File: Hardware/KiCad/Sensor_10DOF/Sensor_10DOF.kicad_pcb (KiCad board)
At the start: 2 copper layers, 38.5 x 30.1 mm, 24 parts, among them J1 Conn_01x04, U1 BMI160, U2 BME280, U3 LSM303AGR, U4 WeMos_D1_mini, U6 LP2985-3.3

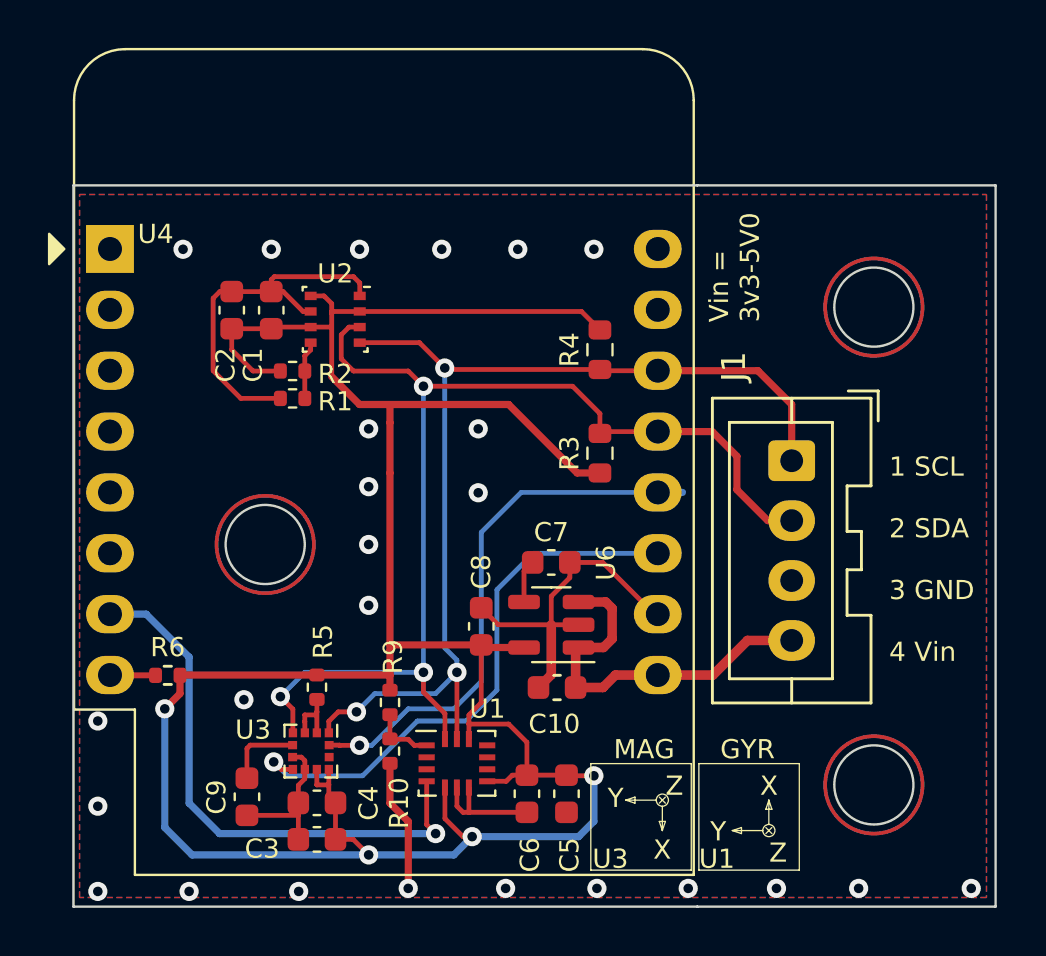
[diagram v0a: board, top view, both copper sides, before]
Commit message: fix gerber
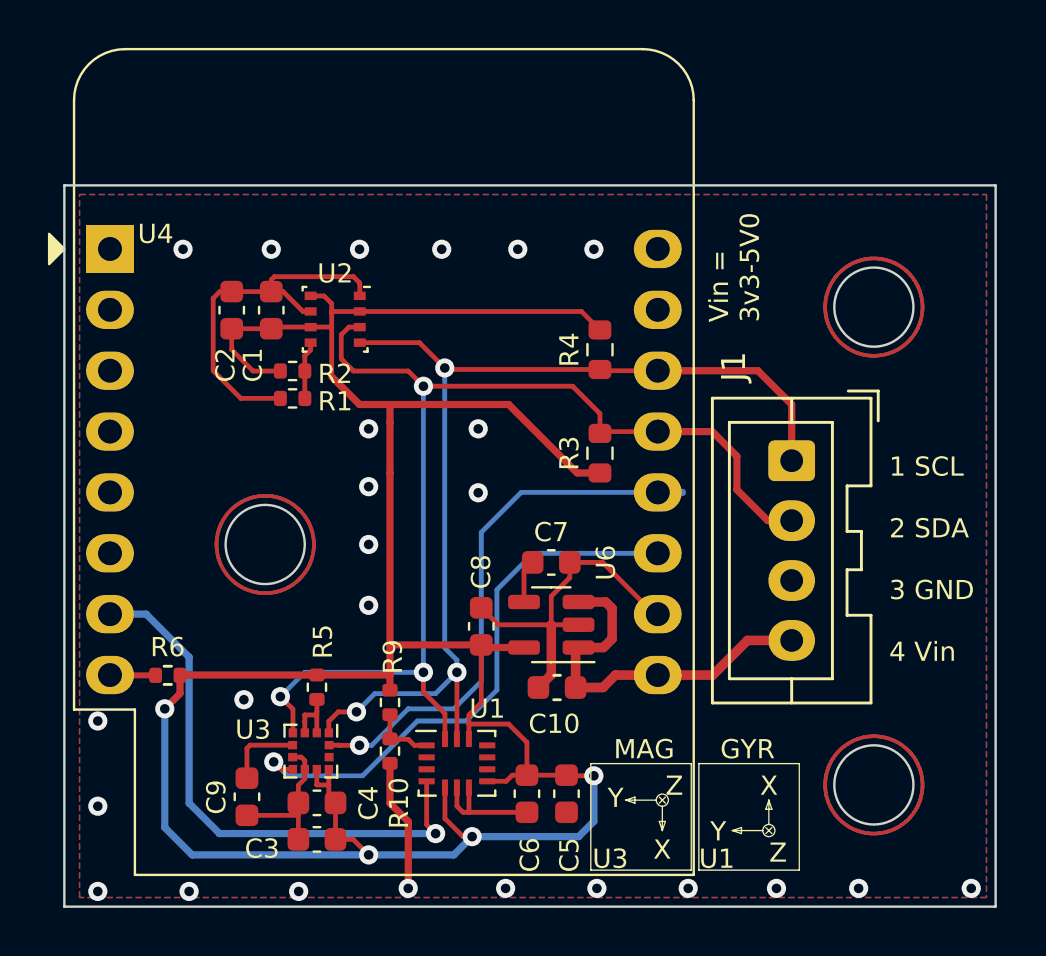
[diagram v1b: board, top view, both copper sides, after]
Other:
- board size 38.5 x 30.1 mm -> 38.9 x 30.1 mm
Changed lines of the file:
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@@
     (pad_to_mask_clearance 0)
     (pcbplotparams
-      (layerselection 0x00010fc_ffffffff)
+      (layerselection 0x0000000_7fffffff)
       (plot_on_all_layers_selection 0x0001120_00000001)
       (disableapertmacros false)
@@
       (sketchpadsonfab false)
       (subtractmaskfromsilk true)
-      (outputformat 1)
+      (outputformat 4)
       (mirror false)
       (drillshape 0)
       (scaleselection 1)
-      (outputdirectory "gerber/")
+      (outputdirectory "./")
     )
   )
@@
     (property "ki_description" "Resistor")
     (property "ki_keywords" "R res resistor")
-    (attr smd)
+    (attr smd exclude_from_pos_files exclude_from_bom allow_missing_courtyard)
     (fp_text reference "R2" (at 1.778 0.127) (layer "F.SilkS")
         (effects (font (size 0.8 0.8) (thickness 0.15)))
@@
     (property "ki_description" "32-bit microcontroller module with WiFi")
     (property "ki_keywords" "ESP8266 WiFi microcontroller ESP8266EX")
-    (attr through_hole)
+    (attr through_hole exclude_from_pos_files exclude_from_bom allow_missing_courtyard)
     (fp_text reference "U4" (at 1.905 -0.622) (layer "F.SilkS")
         (effects (font (size 0.8 0.8) (thickness 0.15)))
@@
     (property "ki_description" "Resistor")
     (property "ki_keywords" "R res resistor")
-    (attr smd)
+    (attr smd exclude_from_pos_files exclude_from_bom allow_missing_courtyard)
     (fp_text reference "R9" (at -1.905 -0.127 90) (layer "F.SilkS")
         (effects (font (size 0.8 0.8) (thickness 0.15)))
@@
     (property "ki_description" "Resistor")
     (property "ki_keywords" "R res resistor")
-    (attr smd)
+    (attr smd exclude_from_pos_files exclude_from_bom allow_missing_courtyard)
     (fp_text reference "R6" (at 0 -1.17) (layer "F.SilkS")
         (effects (font (size 0.8 0.8) (thickness 0.15)))
@@
     (property "ki_description" "Generic connector, single row, 01x04, script generated (kicad-library-utils/schlib/autogen/connector/)")
     (property "ki_keywords" "connector")
-    (attr through_hole)
+    (attr through_hole exclude_from_pos_files exclude_from_bom allow_missing_courtyard)
     (fp_text reference "J1" (at -3.93 2.413 90) (layer "F.SilkS")
         (effects (font (size 1 1) (thickness 0.15)))
@@
   (gr_circle (center 109.982 96.774) (end 109.982 95.123)
     (stroke (width 0.1) (type default)) (fill none) (layer "Edge.Cuts"))
-  (gr_line (start 128.016 111.887) (end 101.981 111.887)
+  (gr_line (start 140.462 111.887) (end 101.6 111.887)
     (stroke (width 0.1) (type default)) (layer "Edge.Cuts"))
-  (gr_line (start 101.981 81.788) (end 128.016 81.788)
-    (stroke (width 0.1) (type default)) (layer "Edge.Cuts"))
-  (gr_line (start 128.016 111.887) (end 140.462 111.887)
+  (gr_line (start 101.6 81.788) (end 140.462 81.788)
     (stroke (width 0.1) (type default)) (layer "Edge.Cuts"))
   (gr_circle (center 135.382 106.807) (end 137.033 106.807)
@@
   (gr_line (start 140.462 81.788) (end 140.462 111.887)
     (stroke (width 0.1) (type default)) (layer "Edge.Cuts"))
-  (gr_line (start 101.981 111.887) (end 101.981 81.788)
-    (stroke (width 0.1) (type default)) (layer "Edge.Cuts"))
-  (gr_line (start 128.016 81.788) (end 140.462 81.788)
+  (gr_line (start 101.6 111.887) (end 101.6 81.788)
     (stroke (width 0.1) (type default)) (layer "Edge.Cuts"))
   (gr_text "VBUS\n\nGND\n\nINT_M\n\nINT_XL\n\nSDA\n\nSCL\n\nRXD\n\nTXD\n" (at 121.412 83.693 180) (layer "B.SilkS")
@@
   )
   (dimension (type aligned) (layer "Dwgs.User")
-    (pts (xy 109.982 96.774) (xy 109.982 81.788))
-    (height -11.684)
-    (gr_text "14.99 mm" (at 97.148 89.281 90) (layer "Dwgs.User")
+    (pts (xy 140.462 81.788) (xy 140.462 111.887))
+    (height -7.493)
+    (gr_text "30.10 mm" (at 146.805 96.8375 90) (layer "Dwgs.User")
       (effects (font (size 1 1) (thickness 0.15)))
     )
@@
   )
   (dimension (type aligned) (layer "Dwgs.User")
-    (pts (xy 109.982 96.774) (xy 101.981 96.774))
-    (height 26.67)
-    (gr_text "8.00 mm" (at 105.9815 68.954) (layer "Dwgs.User")
+    (pts (xy 109.982 96.774) (xy 109.982 81.788))
+    (height -11.049)
+    (gr_text "14.99 mm" (at 97.783 89.281 90) (layer "Dwgs.User")
       (effects (font (size 1 1) (thickness 0.15)))
     )
@@
   )
   (dimension (type aligned) (layer "Dwgs.User")
-    (pts (xy 101.981 81.788) (xy 140.462 81.788))
-    (height -8.001)
-    (gr_text "38.4810 mm" (at 121.2215 71.987) (layer "Dwgs.User")
-      (effects (font (size 1.5 1.5) (thickness 0.3)))
-    )
-    (format (prefix "") (suffix "") (units 3) (units_format 1) (precision 4))
-    (style (thickness 0.2) (arrow_length 1.27) (text_position_mode 0) (extension_height 0.58642) (extension_offset 0.5) keep_text_aligned)
+    (pts (xy 135.382 86.868) (xy 140.462 86.868))
+    (height -7.874)
+    (gr_text "5.08 mm" (at 139.954 77.724) (layer "Dwgs.User")
+      (effects (font (size 1 1) (thickness 0.15)))
+    )
+    (format (prefix "") (suffix "") (units 3) (units_format 1) (precision 2))
+    (style (thickness 0.15) (arrow_length 1.27) (text_position_mode 2) (extension_height 0.58642) (extension_offset 0.5) keep_text_aligned)
+  )
+  (dimension (type aligned) (layer "Dwgs.User")
+    (pts (xy 101.6 81.788) (xy 140.462 81.788))
+    (height -10.033)
+    (gr_text "38.86 mm" (at 121.031 70.605) (layer "Dwgs.User")
+      (effects (font (size 1 1) (thickness 0.15)))
+    )
+    (format (prefix "") (suffix "") (units 3) (units_format 1) (precision 2))
+    (style (thickness 0.15) (arrow_length 1.27) (text_position_mode 0) (extension_height 0.58642) (extension_offset 0.5) keep_text_aligned)
+  )
+  (dimension (type aligned) (layer "Dwgs.User")
+    (pts (xy 109.982 96.774) (xy 101.6 96.774))
+    (height 21.971)
+    (gr_text "8.38 mm" (at 105.791 73.653) (layer "Dwgs.User")
+      (effects (font (size 1 1) (thickness 0.15)))
+    )
+    (format (prefix "") (suffix "") (units 3) (units_format 1) (precision 2))
+    (style (thickness 0.15) (arrow_length 1.27) (text_position_mode 0) (extension_height 0.58642) (extension_offset 0.5) keep_text_aligned)
   )
   (dimension (type aligned) (layer "Dwgs.User")
     (pts (xy 135.382 86.868) (xy 135.382 81.788))
     (height 8.636)
-    (gr_text "5.08 mm" (at 143.891 77.978 90) (layer "Dwgs.User")
+    (gr_text "5.08 mm" (at 142.621 82.296 90) (layer "Dwgs.User")
       (effects (font (size 1 1) (thickness 0.15)))
     )
-    (format (prefix "") (suffix "") (units 3) (units_format 1) (precision 2))
-    (style (thickness 0.15) (arrow_length 1.27) (text_position_mode 2) (extension_height 0.58642) (extension_offset 0.5) keep_text_aligned)
-  )
-  (dimension (type aligned) (layer "Dwgs.User")
-    (pts (xy 135.382 86.868) (xy 140.462 86.868))
-    (height -8.89)
-    (gr_text "5.08 mm" (at 138.43 76.581) (layer "Dwgs.User")
-      (effects (font (size 1 1) (thickness 0.15)))
-    )
-    (format (prefix "") (suffix "") (units 3) (units_format 1) (precision 2))
-    (style (thickness 0.15) (arrow_length 1.27) (text_position_mode 2) (extension_height 0.58642) (extension_offset 0.5) keep_text_aligned)
-  )
-  (dimension (type aligned) (layer "Dwgs.User")
-    (pts (xy 135.382 106.807) (xy 140.462 106.807))
-    (height 9.525)
-    (gr_text "5.08 mm" (at 138.049 118.364) (layer "Dwgs.User")
-      (effects (font (size 1 1) (thickness 0.15)))
-    )
-    (format (prefix "") (suffix "") (units 3) (units_format 1) (precision 2))
-    (style (thickness 0.15) (arrow_length 1.27) (text_position_mode 2) (extension_height 0.58642) (extension_offset 0.5) keep_text_aligned)
-  )
-  (dimension (type aligned) (layer "Dwgs.User")
-    (pts (xy 140.462 111.887) (xy 140.462 81.788))
-    (height 6.858)
-    (gr_text "30.0990 mm" (at 146.17 96.8375 90) (layer "Dwgs.User")
-      (effects (font (size 1 1) (thickness 0.15)))
-    )
-    (format (prefix "") (suffix "") (units 3) (units_format 1) (precision 4))
-    (style (thickness 0.15) (arrow_length 1.27) (text_position_mode 0) (extension_height 0.58642) (extension_offset 0.5) keep_text_aligned)
-  )
-  (dimension (type aligned) (layer "Dwgs.User")
-    (pts (xy 135.382 106.807) (xy 135.382 111.887))
-    (height -8.509)
-    (gr_text "5.08 mm" (at 145.542 108.331 90) (layer "Dwgs.User")
-      (effects (font (size 1 1) (thickness 0.15)))
-    )

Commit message: bestückungsplan erstellt
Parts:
- R2, R6, R9: value N.P. -> DNP
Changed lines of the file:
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@@
     (pad_to_mask_clearance 0)
     (pcbplotparams
-      (layerselection 0x0000000_7fffffff)
-      (plot_on_all_layers_selection 0x0001120_00000001)
+      (layerselection 0x0000020_7ffffffe)
+      (plot_on_all_layers_selection 0x0001020_00000000)
       (disableapertmacros false)
       (usegerberextensions true)
@@
         (effects (font (size 0.8 0.8) (thickness 0.15)))
     )
-    (fp_text value "10uF" (at 0 1.43) (layer "F.Fab")
+    (fp_text value "10uF" (at -3.048 -0.013) (layer "F.Fab")
         (effects (font (size 0.8 0.8) (thickness 0.15)))
     )
@@
         (effects (font (size 0.8 0.8) (thickness 0.15)))
     )
-    (fp_text value "0R0" (at 0 1.17) (layer "F.Fab")
+    (fp_text value "0R0" (at 2.159 1.016) (layer "F.Fab")
         (effects (font (size 0.8 0.8) (thickness 0.15)))
     )
@@
         (effects (font (size 0.8 0.8) (thickness 0.15)))
     )
-    (fp_text value "LP2985-3.3" (at 0 2.4) (layer "F.Fab")
+    (fp_text value "LP2985-3.3" (at 5.588 2.334) (layer "F.Fab")
         (effects (font (size 0.8 0.8) (thickness 0.15)))
     )
@@
         (effects (font (size 0.8 0.8) (thickness 0.15)))
     )
-    (fp_text value "10nF" (at 0 1.43) (layer "F.Fab")
+    (fp_text value "10nF" (at 0 -1.257) (layer "F.Fab")
         (effects (font (size 0.8 0.8) (thickness 0.15)))
     )
@@
     (property "ki_description" "Resistor")
     (property "ki_keywords" "R res resistor")
-    (attr smd exclude_from_pos_files exclude_from_bom allow_missing_courtyard)
+    (attr smd exclude_from_pos_files allow_missing_courtyard)
     (fp_text reference "R2" (at 1.778 0.127) (layer "F.SilkS")
         (effects (font (size 0.8 0.8) (thickness 0.15)))
     )
-    (fp_text value "N.P." (at 0 1.17) (layer "F.Fab")
+    (fp_text value "DNP" (at -2.159 1.27) (layer "F.Fab")
         (effects (font (size 0.8 0.8) (thickness 0.15)))
     )
@@
     (property "ki_description" "32-bit microcontroller module with WiFi")
     (property "ki_keywords" "ESP8266 WiFi microcontroller ESP8266EX")
-    (attr through_hole exclude_from_pos_files exclude_from_bom allow_missing_courtyard)
+    (attr through_hole exclude_from_pos_files allow_missing_courtyard)
     (fp_text reference "U4" (at 1.905 -0.622) (layer "F.SilkS")
         (effects (font (size 0.8 0.8) (thickness 0.15)))
     )
-    (fp_text value "WeMos_D1_mini" (at 11.7 0) (layer "F.Fab")
+    (fp_text value "WeMos_D1_mini" (at 8.128 -0.876) (layer "F.Fab")
         (effects (font (size 0.8 0.8) (thickness 0.15)))
     )
@@
         (effects (font (size 0.8 0.8) (thickness 0.15)))
     )
-    (fp_text user "${REFERENCE}" (at 11.43 10) (layer "F.Fab")
+    (fp_text user "${REFERENCE}" (at 1.905 -0.876) (layer "F.Fab")
         (effects (font (size 0.8 0.8) (thickness 0.15)))
     )
@@
         (effects (font (size 0.8 0.8) (thickness 0.15)))
     )
-    (fp_text value "1u" (at 0 1.43) (layer "F.Fab")
+    (fp_text value "1u" (at -2.426 -0.508) (layer "F.Fab")
         (effects (font (size 1 1) (thickness 0.15)))
     )
@@
         (effects (font (size 0.8 0.8) (thickness 0.15)))
     )
-    (fp_text value "0R0" (at 2.286 -0.127 90) (layer "F.Fab") hide
+    (fp_text value "0R0" (at 0.14 0.889 90) (layer "F.Fab")
         (effects (font (size 0.8 0.8) (thickness 0.15)))
     )
@@
         (effects (font (size 0.8 0.8) (thickness 0.15)))
     )
-    (fp_text value "100nF" (at 0 1.43 90) (layer "F.Fab")
+    (fp_text value "100nF" (at 0.127 -1.397 90) (layer "F.Fab")
         (effects (font (size 0.8 0.8) (thickness 0.15)))
     )
@@
     (property "ki_description" "Resistor")
     (property "ki_keywords" "R res resistor")
-    (attr smd exclude_from_pos_files exclude_from_bom allow_missing_courtyard)
+    (attr smd exclude_from_pos_files allow_missing_courtyard)
     (fp_text reference "R9" (at -1.905 -0.127 90) (layer "F.SilkS")
         (effects (font (size 0.8 0.8) (thickness 0.15)))
     )
-    (fp_text value "N.P." (at 0 1.17 90) (layer "F.Fab") hide
+    (fp_text value "DNP" (at -1.511 0.889 -90) (layer "F.Fab")
         (effects (font (size 0.8 0.8) (thickness 0.15)))
     )
@@
         (effects (font (size 0.8 0.8) (thickness 0.15)))
     )
-    (fp_text value "0R0" (at 0 1.17 90) (layer "F.Fab")
+    (fp_text value "0R0" (at -2.146 -0.127 90) (layer "F.Fab")
         (effects (font (size 0.8 0.8) (thickness 0.15)))
     )
@@
         (effects (font (size 0.8 0.8) (thickness 0.15)))
     )
-    (fp_text value "220nF" (at 0 1.43 90) (layer "F.Fab")
+    (fp_text value "220nF" (at 0 1.27 90) (layer "F.Fab")
         (effects (font (size 0.8 0.8) (thickness 0.15)))
     )
@@
         (effects (font (size 0.8 0.8) (thickness 0.15)))
     )
-    (fp_text value "100nF" (at 0 1.43 90) (layer "F.Fab")
+    (fp_text value "100nF" (at 2.299 0) (layer "F.Fab")
         (effects (font (size 0.8 0.8) (thickness 0.15)))
     )
@@
     (property "ki_description" "Resistor")
     (property "ki_keywords" "R res resistor")
-    (attr smd exclude_from_pos_files exclude_from_bom allow_missing_courtyard)
+    (attr smd exclude_from_pos_files allow_missing_courtyard)
     (fp_text reference "R6" (at 0 -1.17) (layer "F.SilkS")
         (effects (font (size 0.8 0.8) (thickness 0.15)))
     )
-    (fp_text value "N.P." (at 0 1.17) (layer "F.Fab")
-        (effects (font (size 1 1) (thickness 0.15)))
+    (fp_text value "DNP" (at 2.415 -0.381) (layer "F.Fab")
+        (effects (font (size 0.8 0.8) (thickness 0.15)))
     )
     (fp_text user "${REFERENCE}" (at 0 0) (layer "F.Fab")
@@
         (effects (font (size 0.8 0.8) (thickness 0.15)))
     )
-    (fp_text value "BMI160" (at 0 2.5) (layer "F.Fab")
+    (fp_text value "BMI160" (at 0.381 -2.019) (layer "F.Fab")
         (effects (font (size 0.8 0.8) (thickness 0.15)))
     )
@@
         (effects (font (size 0.8 0.8) (thickness 0.15)))
     )
-    (fp_text value "4K7" (at 0 1.43 90) (layer "F.Fab")
+    (fp_text value "4K7" (at 0 -1.27 90) (layer "F.Fab")
         (effects (font (size 0.8 0.8) (thickness 0.15)))
     )
@@
     (property "ki_description" "Generic connector, single row, 01x04, script generated (kicad-library-utils/schlib/autogen/connector/)")
     (property "ki_keywords" "connector")
-    (attr through_hole exclude_from_pos_files exclude_from_bom allow_missing_courtyard)
+    (attr through_hole exclude_from_pos_files allow_missing_courtyard)
     (fp_text reference "J1" (at -3.93 2.413 90) (layer "F.SilkS")
         (effects (font (size 1 1) (thickness 0.15)))
     )
-    (fp_text value "Conn_01x04" (at 3.75 4.4 90) (layer "F.Fab")
+    (fp_text value "Conn_01x04" (at 3.877 -4.572 90) (layer "F.Fab")
         (effects (font (size 1 1) (thickness 0.15)))
     )
@@
         (effects (font (size 0.8 0.8) (thickness 0.15)))
     )
-    (fp_text value "100nF" (at 0 1.43 90) (layer "F.Fab")
+    (fp_text value "100nF" (at -2.019 -0.381 -180) (layer "F.Fab")
         (effects (font (size 0.8 0.8) (thickness 0.15)))
     )
@@
         (effects (font (size 0.8 0.8) (thickness 0.15)))
     )
-    (fp_text value "BME280" (at 0.015 2.535 90) (layer "F.Fab")
+    (fp_text value "BME280" (at 0.127 -2.54 90) (layer "F.Fab")
         (effects (font (size 0.8 0.8) (thickness 0.15)))
     )
@@
         (effects (font (size 0.8 0.8) (thickness 0.15)))
     )
-    (fp_text value "100nF" (at 0 1.43) (layer "F.Fab")
+    (fp_text value "100nF" (at -3.302 -0.013) (layer "F.Fab")
         (effects (font (size 0.8 0.8) (thickness 0.15)))
     )
@@
         (effects (font (size 0.8 0.8) (thickness 0.15)))
     )
-    (fp_text value "100nF" (at 0 1.43 90) (layer "F.Fab")
+    (fp_text value "100nF" (at 1.905 0.762 180) (layer "F.Fab")
         (effects (font (size 0.8 0.8) (thickness 0.15)))
     )
@@
         (effects (font (size 0.8 0.8) (thickness 0.15)))
     )
-    (fp_text value "4u7" (at 0 1.43 90) (layer "F.Fab")
-        (effects (font (size 0.8 0.8) (thickness 0.15)))
-    )
+    (fp_text value "4u7" (at 0.114 -1.524 90) (layer "F.Fab")
+        (effects (font (size 0.8 0.8) (thickness 0.15)))
+    )
